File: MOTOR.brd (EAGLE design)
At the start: 39.8 x 21.5 mm, 10 parts, among them IC1 BCP56, J1 CONECTOR_MACHO, J2 CONECTOR_FEMEA, U1 74HC132

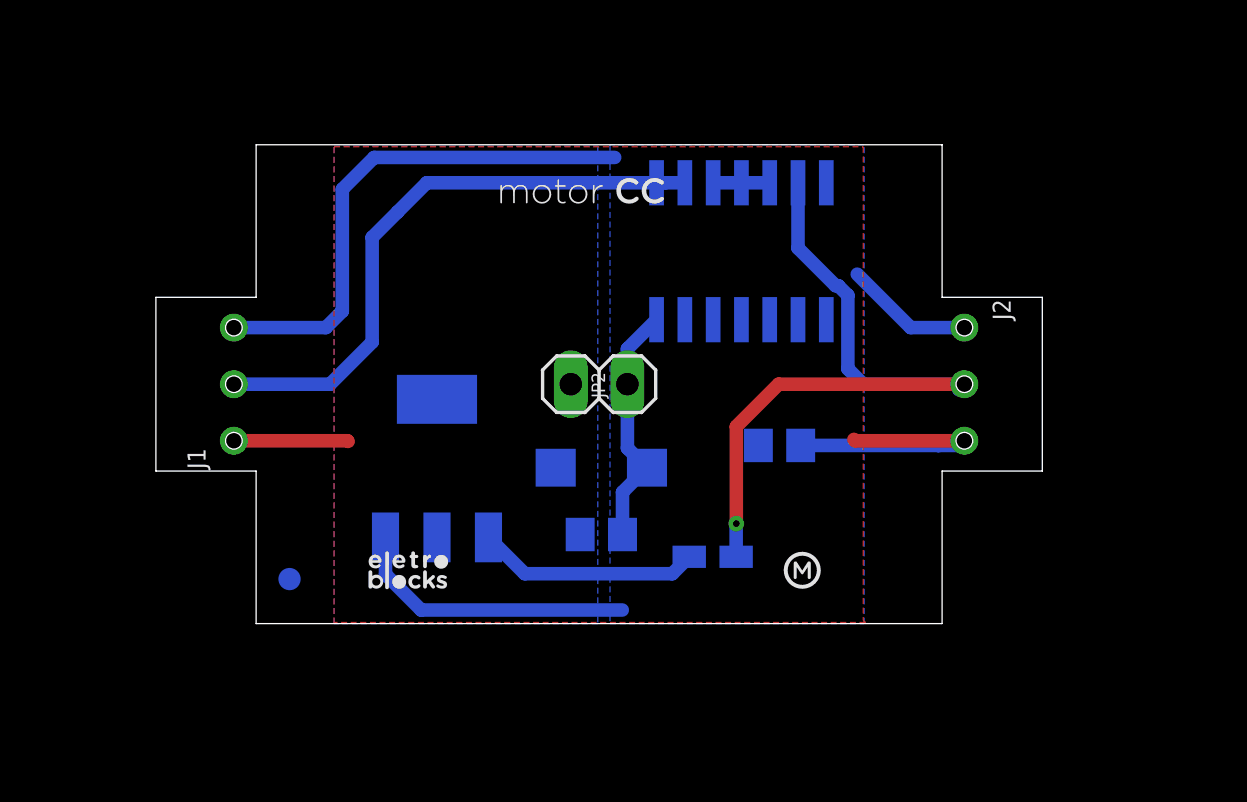
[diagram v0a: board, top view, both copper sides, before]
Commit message: V1.0.2
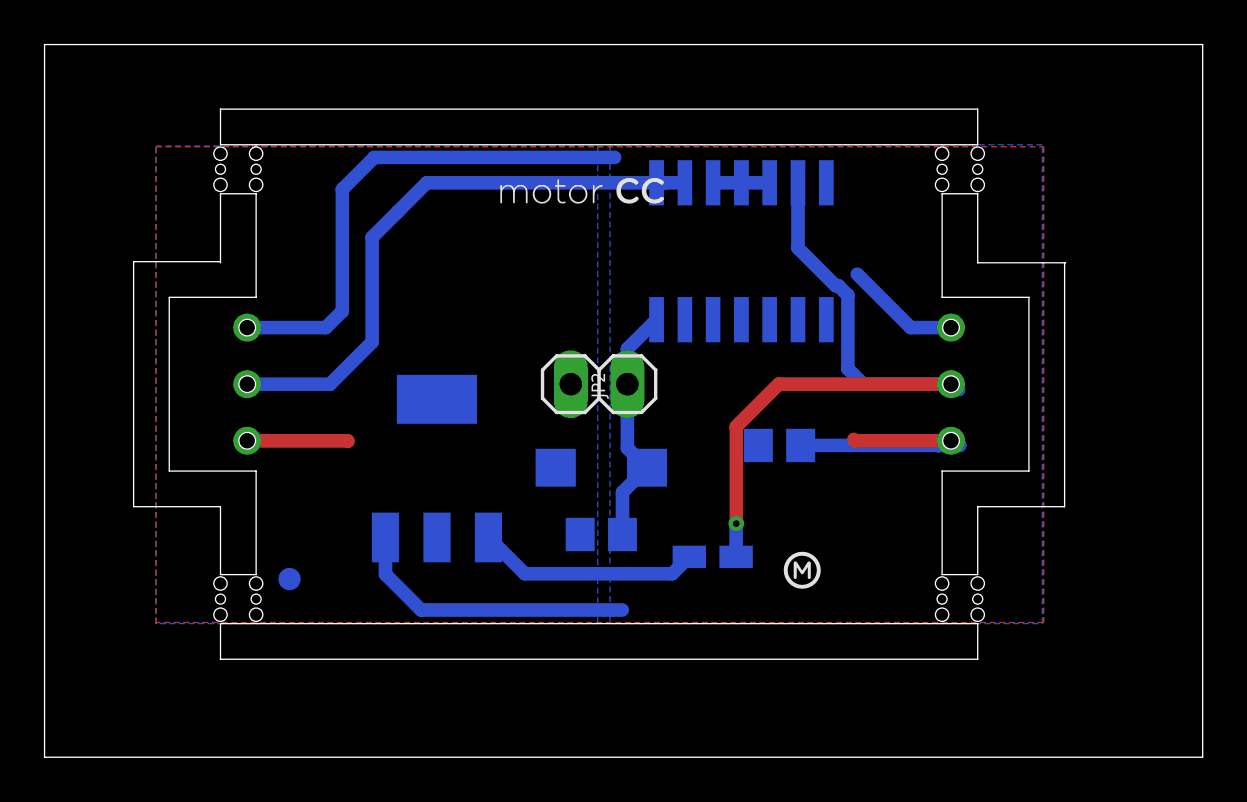
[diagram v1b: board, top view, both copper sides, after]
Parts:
- added U$2, U$3, U$4, U$5: (no value), Eletroblocks Lib:STAMP_DUPLO
- J1: device Eletroblocks Lib:3CONECTOR -> Eletroblocks Lib:MALE
- J2: device Eletroblocks Lib:3CONECTOR -> Eletroblocks Lib:FEMALE
- moved J2 0.60 mm to (27.7, 10.8)
- moved J1 0.60 mm to (-3.90, 10.8)
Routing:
- net GND: track 42.2 -> 41.0 mm
- net SIGNAL_OUT: track 32.1 -> 31.0 mm
- net VCC: track 28.6 -> 27.5 mm
- net SIGNAL_IN: track 26.7 -> 26.1 mm
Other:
- board size 39.8 x 21.5 mm -> 52 x 32 mm
- board text added: "V1.0.2"
- board text removed: "V1.0.1"
